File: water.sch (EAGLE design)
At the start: 21 parts, among them K1 AQH2223, K2 AQH2223, K3 AQH2223, K4 AQH2223, X5 MKDSN1,5/2-5,08, X6 MKDSN1,5/2-5,08, X7 MKDSN1,5/2-5,08, X8 MKDSN1,5/2-5,08

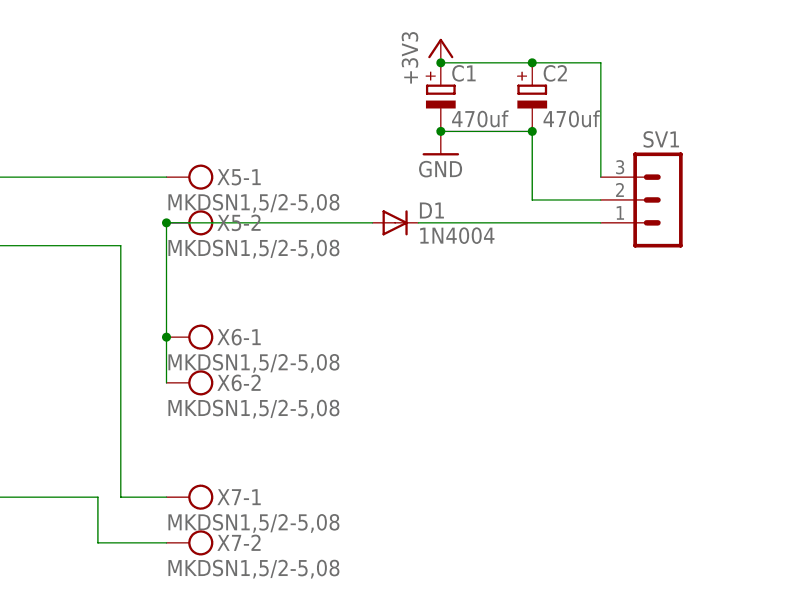
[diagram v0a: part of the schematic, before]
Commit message: More features
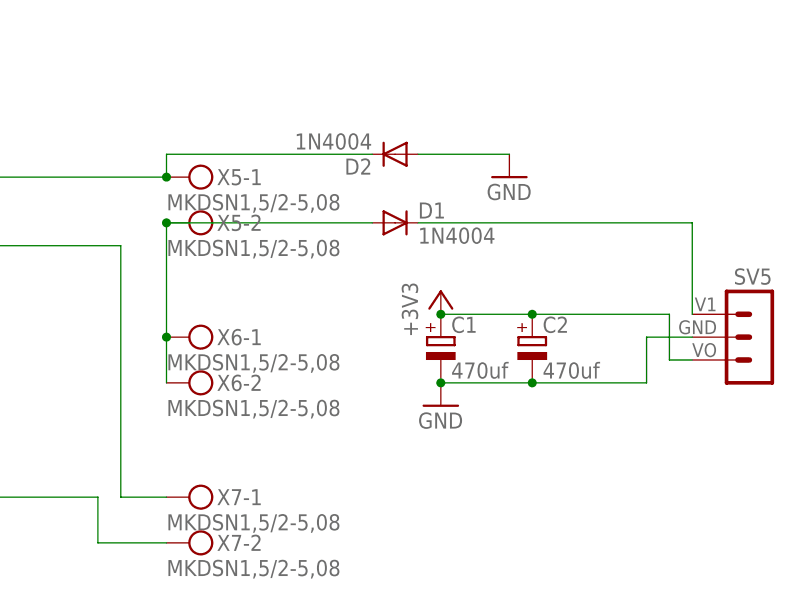
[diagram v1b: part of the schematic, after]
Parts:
- removed SV1: (no value), con-lstb:MA03-1
- added D2: 1N4004, diode:1N4004
- added SV5: (no value), my-parts:DC-DC3V3
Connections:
- net +3V3: now also SV5.VO; no longer SV1.3
- net GND: now also D2.A, SV5.GND; no longer SV1.2
- net N$14: now also SV5.V1; no longer SV1.1
- net N$21: now also D2.C
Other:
- moved on the sheet: C1, C2
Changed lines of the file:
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@@
 <part name="GND4" library="supply1" library_urn="urn:adsk.eagle:library:371" deviceset="GND" device=""/>
 <part name="U2" library="esp8266modules" deviceset="ESP12E" device="SMD"/>
-<part name="SV1" library="con-lstb" library_urn="urn:adsk.eagle:library:162" deviceset="MA03-1" device=""/>
 <part name="GND5" library="supply1" library_urn="urn:adsk.eagle:library:371" deviceset="GND" device=""/>
 <part name="+3V1" library="supply1" library_urn="urn:adsk.eagle:library:371" deviceset="+3V3" device=""/>
@@
 <part name="SV3" library="con-lstb" library_urn="urn:adsk.eagle:library:162" deviceset="MA08-1" device=""/>
 <part name="SV4" library="con-lstb" library_urn="urn:adsk.eagle:library:162" deviceset="MA08-1" device=""/>
+<part name="SV5" library="my-parts" deviceset="DC-DC" device="3V3"/>
+<part name="D2" library="diode" library_urn="urn:adsk.eagle:library:210" deviceset="1N4004" device=""/>
+<part name="GND7" library="supply1" library_urn="urn:adsk.eagle:library:371" deviceset="GND" device=""/>
 </parts>
 <sheets>
@@
 <instance part="GND4" gate="1" x="73.66" y="68.58"/>
 <instance part="U2" gate="G$1" x="35.56" y="53.34"/>
-<instance part="SV1" gate="G$1" x="185.42" y="81.28" rot="MR0"/>
-<instance part="GND5" gate="1" x="160.02" y="86.36"/>
-<instance part="+3V1" gate="G$1" x="160.02" y="99.06"/>
+<instance part="GND5" gate="1" x="160.02" y="58.42"/>
+<instance part="+3V1" gate="G$1" x="160.02" y="71.12"/>
 <instance part="+3V2" gate="G$1" x="5.08" y="45.72"/>
 <instance part="GND6" gate="1" x="55.88" y="40.64"/>
@@
 <instance part="+3V3" gate="G$1" x="43.18" y="93.98"/>
 <instance part="GND8" gate="1" x="48.26" y="83.82"/>
-<instance part="C1" gate="G$1" x="160.02" y="93.98"/>
-<instance part="C2" gate="G$1" x="170.18" y="93.98"/>
+<instance part="C1" gate="G$1" x="160.02" y="66.04"/>
+<instance part="C2" gate="G$1" x="170.18" y="66.04"/>
 <instance part="U1" gate="G$1" x="170.18" y="-12.7"/>
 <instance part="SV3" gate="1" x="144.78" y="-15.24"/>
 <instance part="SV4" gate="1" x="193.04" y="-15.24" rot="MR0"/>
+<instance part="SV5" gate="G$1" x="195.58" y="66.04" rot="MR0"/>
+<instance part="D2" gate="1" x="154.94" y="86.36" rot="R180"/>
+<instance part="GND7" gate="1" x="167.64" y="83.82"/>
 </instances>
 <busses>
@@
 <pinref part="C1" gate="G$1" pin="-"/>
 <pinref part="C2" gate="G$1" pin="-"/>
-<wire x1="160.02" y1="88.9" x2="170.18" y2="88.9" width="0.1524" layer="91"/>
-<junction x="160.02" y="88.9"/>
-<wire x1="170.18" y1="88.9" x2="170.18" y2="81.28" width="0.1524" layer="91"/>
-<junction x="170.18" y="88.9"/>
-<pinref part="SV1" gate="G$1" pin="2"/>
-<wire x1="170.18" y1="81.28" x2="177.8" y2="81.28" width="0.1524" layer="91"/>
+<wire x1="160.02" y1="60.96" x2="170.18" y2="60.96" width="0.1524" layer="91"/>
+<junction x="160.02" y="60.96"/>
+<wire x1="170.18" y1="60.96" x2="182.88" y2="60.96" width="0.1524" layer="91"/>
+<wire x1="182.88" y1="60.96" x2="182.88" y2="66.04" width="0.1524" layer="91"/>
+<junction x="170.18" y="60.96"/>
+<pinref part="SV5" gate="G$1" pin="GND"/>
+<wire x1="182.88" y1="66.04" x2="187.96" y2="66.04" width="0.1524" layer="91"/>
+</segment>
+<segment>
+<pinref part="GND7" gate="1" pin="GND"/>
+<pinref part="D2" gate="1" pin="A"/>
+<wire x1="167.64" y1="86.36" x2="157.48" y2="86.36" width="0.1524" layer="91"/>
 </segment>
 </net>
@@
 <pinref part="+3V1" gate="G$1" pin="+3V3"/>
 <pinref part="C1" gate="G$1" pin="+"/>
-<pinref part="SV1" gate="G$1" pin="3"/>
-<wire x1="177.8" y1="83.82" x2="177.8" y2="96.52" width="0.1524" layer="91"/>
 <pinref part="C2" gate="G$1" pin="+"/>
-<wire x1="177.8" y1="96.52" x2="170.18" y2="96.52" width="0.1524" layer="91"/>
-<wire x1="170.18" y1="96.52" x2="160.02" y2="96.52" width="0.1524" layer="91"/>
-<junction x="170.18" y="96.52"/>
-<junction x="160.02" y="96.52"/>
+<wire x1="170.18" y1="68.58" x2="160.02" y2="68.58" width="0.1524" layer="91"/>
+<junction x="170.18" y="68.58"/>
+<junction x="160.02" y="68.58"/>
+<wire x1="170.18" y1="68.58" x2="185.42" y2="68.58" width="0.1524" layer="91"/>
+<wire x1="185.42" y1="68.58" x2="185.42" y2="63.5" width="0.1524" layer="91"/>
+<pinref part="SV5" gate="G$1" pin="VO"/>
+<wire x1="185.42" y1="63.5" x2="187.96" y2="63.5" width="0.1524" layer="91"/>
 </segment>
 </net>
@@
 <junction x="129.54" y="78.74"/>
 <pinref part="D1" gate="1" pin="A"/>
-</segment>
-</net>
-<net name="N$14" class="0">
-<segment>
-<pinref part="D1" gate="1" pin="C"/>
-<pinref part="SV1" gate="G$1" pin="1"/>
-<wire x1="157.48" y1="78.74" x2="177.8" y2="78.74" width="0.1524" layer="91"/>
 </segment>
 </net>
@@
 <wire x1="109.22" y1="83.82" x2="129.54" y2="83.82" width="0.1524" layer="91"/>
 <junction x="109.22" y="83.82"/>
+<pinref part="D2" gate="1" pin="C"/>
+<wire x1="152.4" y1="86.36" x2="129.54" y2="86.36" width="0.1524" layer="91"/>
+<wire x1="129.54" y1="86.36" x2="129.54" y2="83.82" width="0.1524" layer="91"/>
+<junction x="129.54" y="83.82"/>
 </segment>
 </net>
@@
 </segment>
 </net>
+<net name="N$14" class="0">
+<segment>
+<pinref part="D1" gate="1" pin="C"/>
+<pinref part="SV5" gate="G$1" pin="V1"/>
+<wire x1="157.48" y1="78.74" x2="187.96" y2="78.74" width="0.1524" layer="91"/>
+<wire x1="187.96" y1="78.74" x2="187.96" y2="68.58" width="0.1524" layer="91"/>
+</segment>
+</net>

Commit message: Fix conflicts
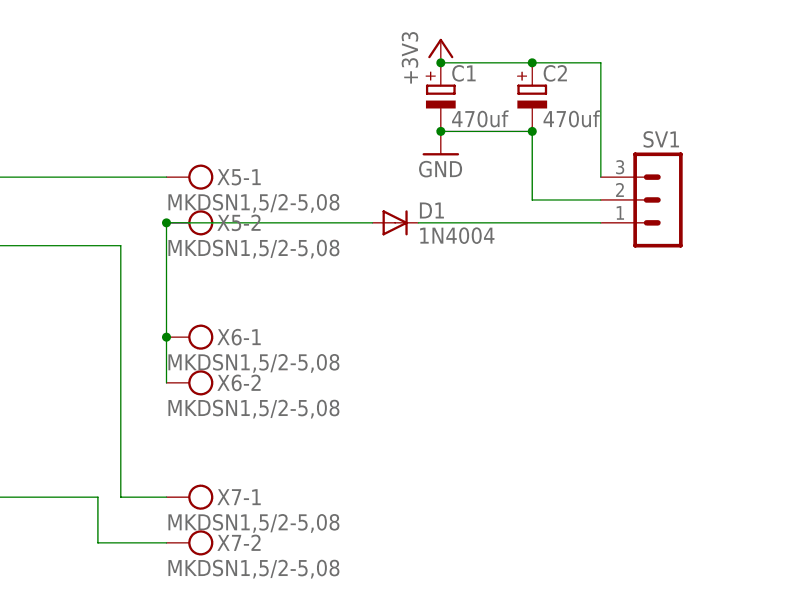
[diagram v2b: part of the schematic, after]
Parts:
- removed D2: 1N4004, diode:1N4004
- removed SV5: (no value), my-parts:DC-DC3V3
- added SV1: (no value), con-lstb:MA03-1
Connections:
- net +3V3: now also SV1.3; no longer SV5.VO
- net GND: now also SV1.2; no longer D2.A, SV5.GND
- net N$14: now also SV1.1; no longer SV5.V1
- net N$21: no longer D2.C
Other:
- moved on the sheet: C1, C2
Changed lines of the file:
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@@
 <part name="GND4" library="supply1" library_urn="urn:adsk.eagle:library:371" deviceset="GND" device=""/>
 <part name="U2" library="esp8266modules" deviceset="ESP12E" device="SMD"/>
+<part name="SV1" library="con-lstb" library_urn="urn:adsk.eagle:library:162" deviceset="MA03-1" device=""/>
 <part name="GND5" library="supply1" library_urn="urn:adsk.eagle:library:371" deviceset="GND" device=""/>
 <part name="+3V1" library="supply1" library_urn="urn:adsk.eagle:library:371" deviceset="+3V3" device=""/>
@@
 <part name="SV3" library="con-lstb" library_urn="urn:adsk.eagle:library:162" deviceset="MA08-1" device=""/>
 <part name="SV4" library="con-lstb" library_urn="urn:adsk.eagle:library:162" deviceset="MA08-1" device=""/>
-<part name="SV5" library="my-parts" deviceset="DC-DC" device="3V3"/>
-<part name="D2" library="diode" library_urn="urn:adsk.eagle:library:210" deviceset="1N4004" device=""/>
-<part name="GND7" library="supply1" library_urn="urn:adsk.eagle:library:371" deviceset="GND" device=""/>
 </parts>
 <sheets>
@@
 <instance part="GND4" gate="1" x="73.66" y="68.58"/>
 <instance part="U2" gate="G$1" x="35.56" y="53.34"/>
-<instance part="GND5" gate="1" x="160.02" y="58.42"/>
-<instance part="+3V1" gate="G$1" x="160.02" y="71.12"/>
+<instance part="SV1" gate="G$1" x="185.42" y="81.28" rot="MR0"/>
+<instance part="GND5" gate="1" x="160.02" y="86.36"/>
+<instance part="+3V1" gate="G$1" x="160.02" y="99.06"/>
 <instance part="+3V2" gate="G$1" x="5.08" y="45.72"/>
 <instance part="GND6" gate="1" x="55.88" y="40.64"/>
@@
 <instance part="+3V3" gate="G$1" x="43.18" y="93.98"/>
 <instance part="GND8" gate="1" x="48.26" y="83.82"/>
-<instance part="C1" gate="G$1" x="160.02" y="66.04"/>
-<instance part="C2" gate="G$1" x="170.18" y="66.04"/>
+<instance part="C1" gate="G$1" x="160.02" y="93.98"/>
+<instance part="C2" gate="G$1" x="170.18" y="93.98"/>
 <instance part="U1" gate="G$1" x="170.18" y="-12.7"/>
 <instance part="SV3" gate="1" x="144.78" y="-15.24"/>
 <instance part="SV4" gate="1" x="193.04" y="-15.24" rot="MR0"/>
-<instance part="SV5" gate="G$1" x="195.58" y="66.04" rot="MR0"/>
-<instance part="D2" gate="1" x="154.94" y="86.36" rot="R180"/>
-<instance part="GND7" gate="1" x="167.64" y="83.82"/>
 </instances>
 <busses>
@@
 <pinref part="C1" gate="G$1" pin="-"/>
 <pinref part="C2" gate="G$1" pin="-"/>
-<wire x1="160.02" y1="60.96" x2="170.18" y2="60.96" width="0.1524" layer="91"/>
-<junction x="160.02" y="60.96"/>
-<wire x1="170.18" y1="60.96" x2="182.88" y2="60.96" width="0.1524" layer="91"/>
-<wire x1="182.88" y1="60.96" x2="182.88" y2="66.04" width="0.1524" layer="91"/>
-<junction x="170.18" y="60.96"/>
-<pinref part="SV5" gate="G$1" pin="GND"/>
-<wire x1="182.88" y1="66.04" x2="187.96" y2="66.04" width="0.1524" layer="91"/>
-</segment>
-<segment>
-<pinref part="GND7" gate="1" pin="GND"/>
-<pinref part="D2" gate="1" pin="A"/>
-<wire x1="167.64" y1="86.36" x2="157.48" y2="86.36" width="0.1524" layer="91"/>
+<wire x1="160.02" y1="88.9" x2="170.18" y2="88.9" width="0.1524" layer="91"/>
+<junction x="160.02" y="88.9"/>
+<wire x1="170.18" y1="88.9" x2="170.18" y2="81.28" width="0.1524" layer="91"/>
+<junction x="170.18" y="88.9"/>
+<pinref part="SV1" gate="G$1" pin="2"/>
+<wire x1="170.18" y1="81.28" x2="177.8" y2="81.28" width="0.1524" layer="91"/>
 </segment>
 </net>
@@
 <pinref part="+3V1" gate="G$1" pin="+3V3"/>
 <pinref part="C1" gate="G$1" pin="+"/>
+<pinref part="SV1" gate="G$1" pin="3"/>
+<wire x1="177.8" y1="83.82" x2="177.8" y2="96.52" width="0.1524" layer="91"/>
 <pinref part="C2" gate="G$1" pin="+"/>
-<wire x1="170.18" y1="68.58" x2="160.02" y2="68.58" width="0.1524" layer="91"/>
-<junction x="170.18" y="68.58"/>
-<junction x="160.02" y="68.58"/>
-<wire x1="170.18" y1="68.58" x2="185.42" y2="68.58" width="0.1524" layer="91"/>
-<wire x1="185.42" y1="68.58" x2="185.42" y2="63.5" width="0.1524" layer="91"/>
-<pinref part="SV5" gate="G$1" pin="VO"/>
-<wire x1="185.42" y1="63.5" x2="187.96" y2="63.5" width="0.1524" layer="91"/>
+<wire x1="177.8" y1="96.52" x2="170.18" y2="96.52" width="0.1524" layer="91"/>
+<wire x1="170.18" y1="96.52" x2="160.02" y2="96.52" width="0.1524" layer="91"/>
+<junction x="170.18" y="96.52"/>
+<junction x="160.02" y="96.52"/>
 </segment>
 </net>
@@
 <junction x="129.54" y="78.74"/>
 <pinref part="D1" gate="1" pin="A"/>
+</segment>
+</net>
+<net name="N$14" class="0">
+<segment>
+<pinref part="D1" gate="1" pin="C"/>
+<pinref part="SV1" gate="G$1" pin="1"/>
+<wire x1="157.48" y1="78.74" x2="177.8" y2="78.74" width="0.1524" layer="91"/>
 </segment>
 </net>
@@
 <wire x1="109.22" y1="83.82" x2="129.54" y2="83.82" width="0.1524" layer="91"/>
 <junction x="109.22" y="83.82"/>
-<pinref part="D2" gate="1" pin="C"/>
-<wire x1="152.4" y1="86.36" x2="129.54" y2="86.36" width="0.1524" layer="91"/>
-<wire x1="129.54" y1="86.36" x2="129.54" y2="83.82" width="0.1524" layer="91"/>
-<junction x="129.54" y="83.82"/>
 </segment>
 </net>
@@
 </segment>
 </net>
-<net name="N$14" class="0">
-<segment>
-<pinref part="D1" gate="1" pin="C"/>
-<pinref part="SV5" gate="G$1" pin="V1"/>
-<wire x1="157.48" y1="78.74" x2="187.96" y2="78.74" width="0.1524" layer="91"/>
-<wire x1="187.96" y1="78.74" x2="187.96" y2="68.58" width="0.1524" layer="91"/>
-</segment>
-</net>
